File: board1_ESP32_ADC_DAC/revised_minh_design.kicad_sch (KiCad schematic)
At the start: 15 parts, among them J1 Conn_01x03_Male, J2 Conn_01x07_Male, U1 ESP32-DevKit-C, U2 LM7805_TO220, U3 NE5532, U4 CB101

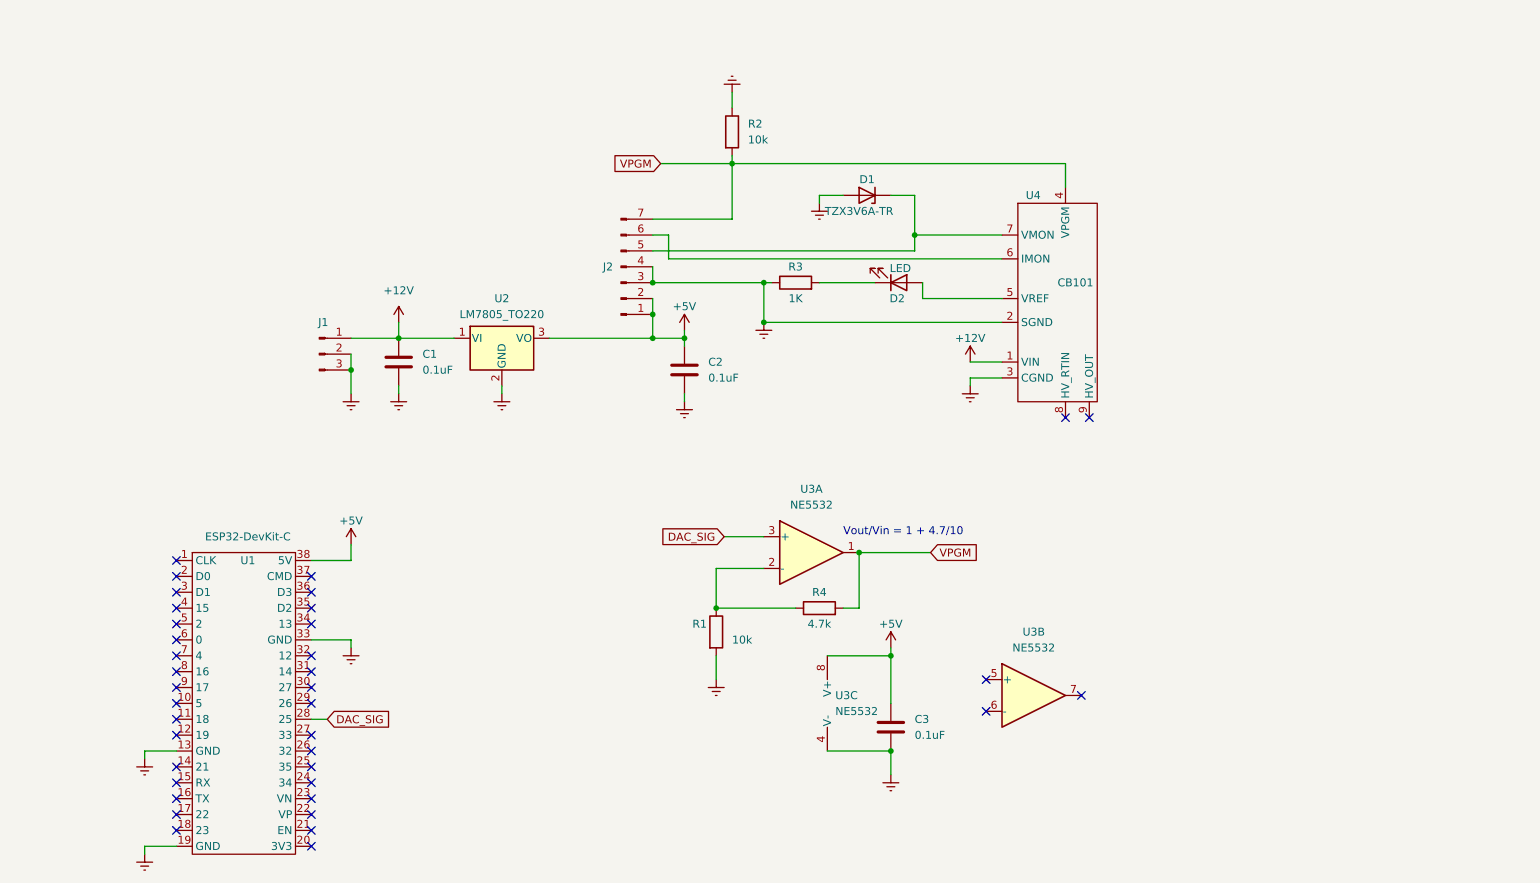
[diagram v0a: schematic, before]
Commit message: -
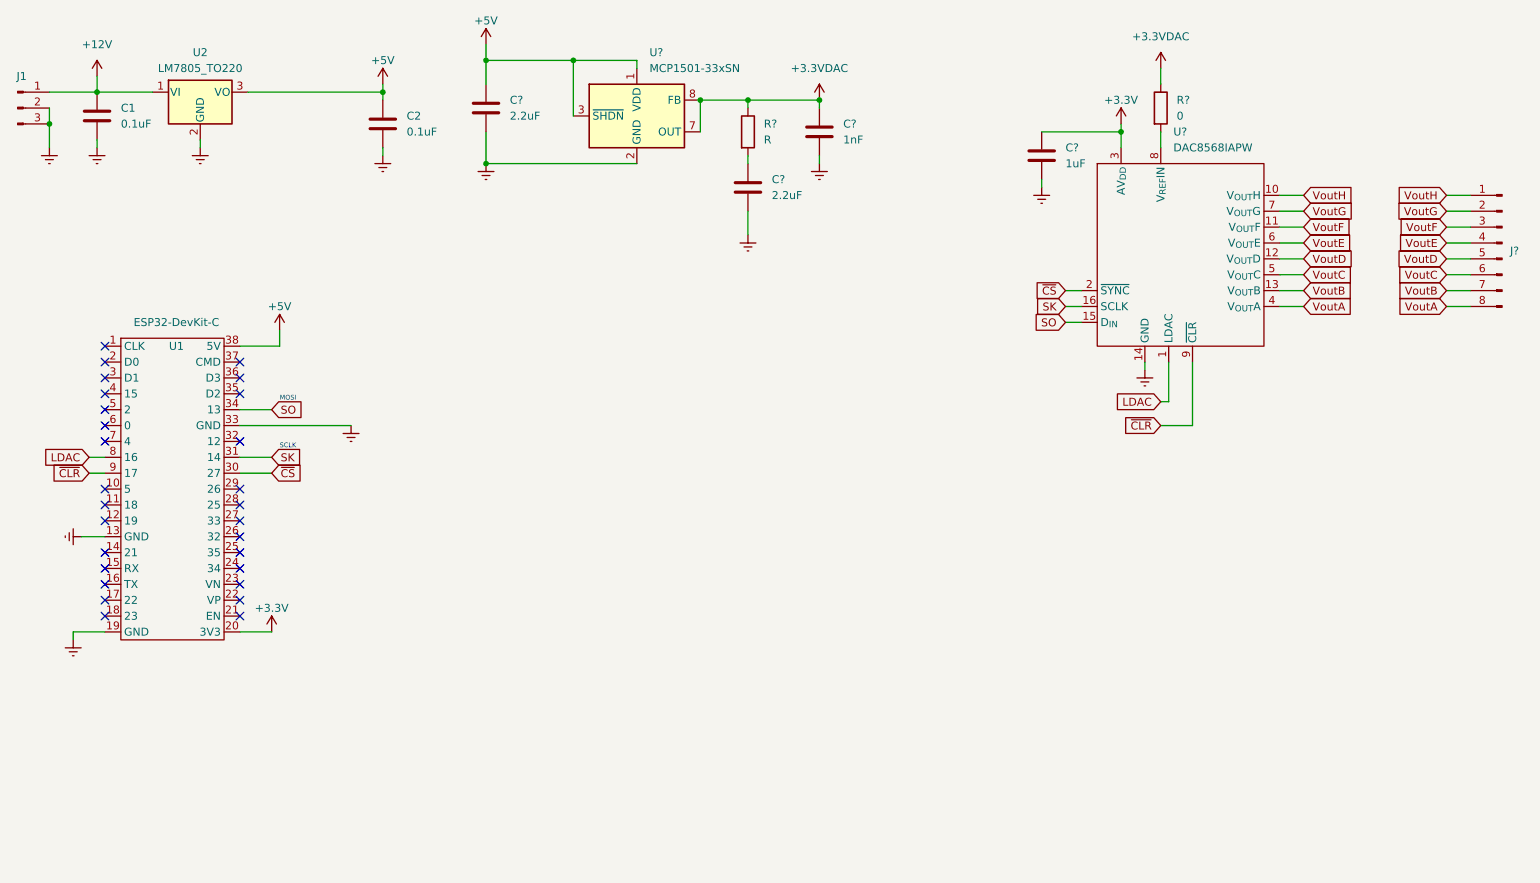
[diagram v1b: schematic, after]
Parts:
- removed C3: 0.1uF, Capacitor_THT:C_Disc_D6.0mm_W2.5mm_P5.00mm, symbol Device:C
- removed D1: TZX3V6A-TR, Diode_THT:D_DO-35_SOD27_P7.62mm_Horizontal, symbol Device:D_Zener
- removed D2: LED, LED_THT:LED_D3.0mm_Clear, symbol Device:LED
- removed J2: Conn_01x07_Male, Connector_PinSocket_2.54mm:PinSocket_1x07_P2.54mm_Vertical, symbol Connector:Conn_01x07_Male
- removed R1, R2: 10k, Resistor_THT:R_Axial_DIN0309_L9.0mm_D3.2mm_P15.24mm_Horizontal, symbol Device:R
- removed R3: 1K, Resistor_THT:R_Axial_DIN0309_L9.0mm_D3.2mm_P15.24mm_Horizontal, symbol Device:R
- removed R4: 4.7k, Resistor_THT:R_Axial_DIN0309_L9.0mm_D3.2mm_P15.24mm_Horizontal, symbol Device:R
- removed U3: NE5532, Package_DIP:DIP-8_W7.62mm, symbol Amplifier_Operational:NE5532
- removed U4: CB101, Library:CB101, symbol design:CB101
- added C? (x2): 2.2uF, Capacitor_THT:C_Disc_D6.0mm_W2.5mm_P5.00mm, symbol Device:C
- added C?: 1uF, Capacitor_THT:C_Disc_D6.0mm_W2.5mm_P5.00mm, symbol Device:C
- added C?: 1nF, Capacitor_THT:C_Disc_D6.0mm_W2.5mm_P5.00mm, symbol Device:C
- added J?: Conn_01x08_Male, symbol Connector:Conn_01x08_Male
- added R?: 0, symbol Device:R
- added R?: R, symbol Device:R
- added U?: DAC8568IAPW, Package_SO:TSSOP-16-1EP_4.4x5mm_P0.65mm, symbol design:DAC8568IAPW
- added U?: MCP1501-33xSN, Package_SO:SOIC-8_3.9x4.9mm_P1.27mm, symbol Reference_Voltage:MCP1501-33xSN
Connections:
- net +5V: now also C?.1, U?.1 (VDD), U?.3 (~{SHDN})
- net Earth: now also C?.2, C?.2, C?.2, C?.2, U?.14 (GND), U?.2 (GND), U?.4 (GND), U?.5 (GND), U?.6 (GND)
- net +3V3: now reaches U1.20 (3V3)
- net +3V3: now also C?.1, U?.3 (AV_{DD})
- net ~{CS}: now reaches U1.30 (27)
- net ~{CS}: now also U?.2 (~{SYNC})
- net SK: now reaches U1.31 (14)
- net SK: now also U?.16 (SCLK)
- net SO: now reaches U1.34 (13)
- net SO: now also U?.15 (D_{IN})
- net LDAC: now reaches U1.8 (16)
- net LDAC: now also U?.1 (LDAC)
- net ~{CLR}: now reaches U1.9 (17)
- net ~{CLR}: now also U?.9 (~{CLR})
- net DAC_SIG: no longer names the net of U1.28 (25)
- new net: C?.1, R?.2
- new net: R?.2, U?.8 (V_{REF}IN)
- new net +3.3VDAC: C?.1, R?.1, R?.1, U?.7 (OUT), U?.8 (FB)
- new net VoutA: J?.8 (Pin_8), U?.4 (V_{OUT}A)
- new net VoutB: J?.7 (Pin_7), U?.13 (V_{OUT}B)
- new net VoutC: J?.6 (Pin_6), U?.5 (V_{OUT}C)
- new net VoutD: J?.5 (Pin_5), U?.12 (V_{OUT}D)
- new net VoutE: J?.4 (Pin_4), U?.6 (V_{OUT}E)
- new net VoutF: J?.3 (Pin_3), U?.11 (V_{OUT}F)
- new net VoutG: J?.2 (Pin_2), U?.7 (V_{OUT}G)
- new net VoutH: J?.1 (Pin_1), U?.10 (V_{OUT}H)
- no-connect marks 38 -> 28
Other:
- note added: "MOSI"
- note added: "SCLK"
- note removed: "Vout/Vin = 1 + 4.7/10"
- moved on the sheet: C1, C2, J1, U1, U2
